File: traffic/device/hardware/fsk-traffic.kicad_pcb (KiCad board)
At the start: 2 copper layers, 83 x 45.5 mm, 49 parts, among them J1 JTAG, J2 USB_C, J3 Molex 5569-04A1, J4 Molex 5569-04A1, J5 Molex 5569-04A1, Q1 MMBT5551, Q2 AO3401A, Q3 MMBT5551, Q4 AO3401A, U1 XC6206P332MR, U2 MT3608, U3 STM32F070F6Px, U4 LTV-817S, U5 LTV-817S, Y1 12MHz

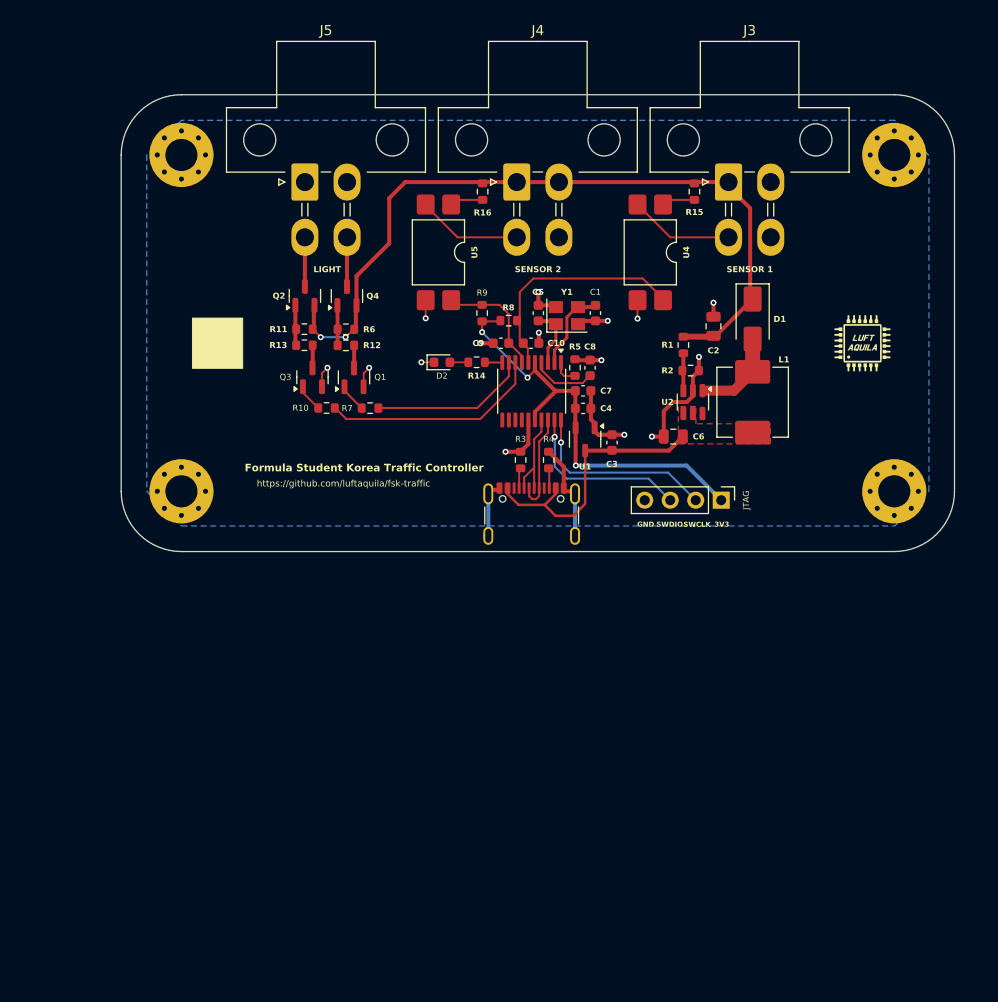
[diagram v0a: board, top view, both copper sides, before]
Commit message: impl: schematic and pcb layout
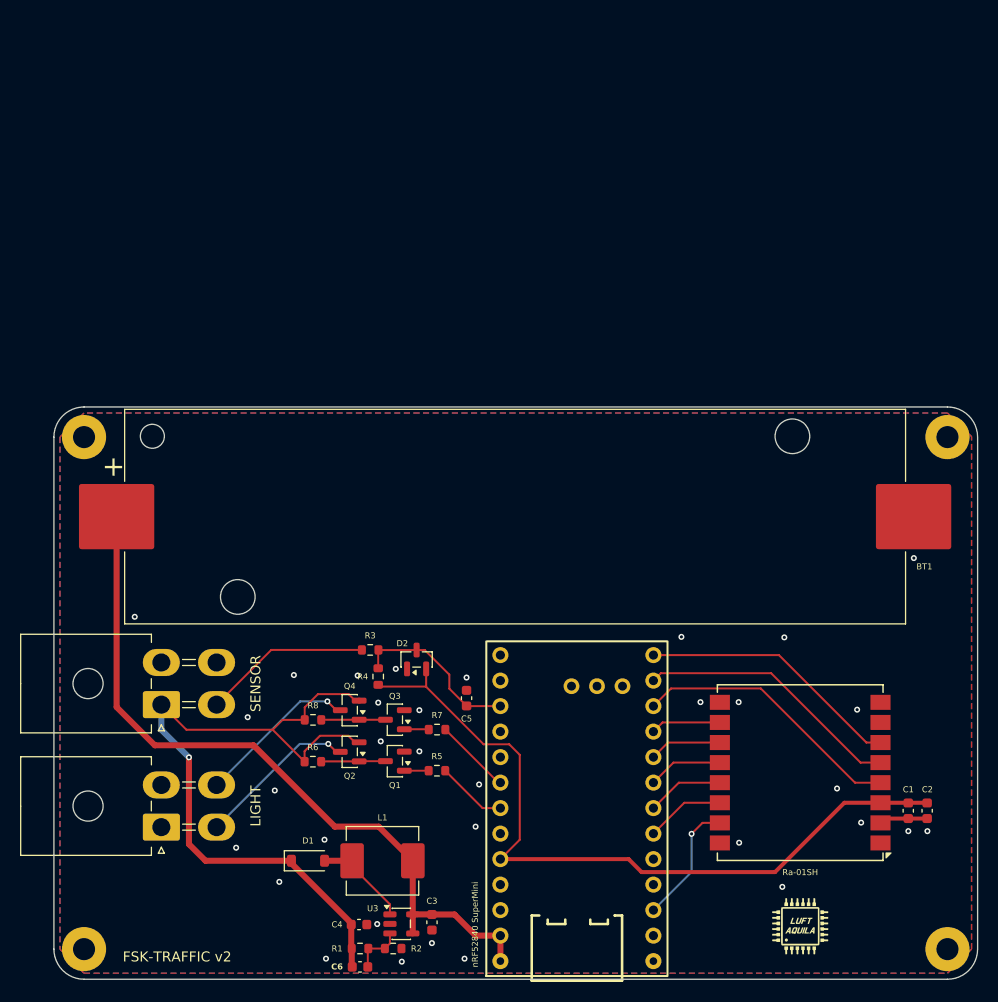
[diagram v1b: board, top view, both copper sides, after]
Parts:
- removed C10, C9: 470nF, Capacitor_SMD:C_0603_1608Metric
- removed C7, C8: 100nF, Capacitor_SMD:C_0603_1608Metric
- removed the G*** at (176.6, 104.6)
- removed J3, J4, J5: Molex 5569-04A1, Connector_Molex:Molex_Mini-Fit_Jr_5569-04A1_2x02_P4.20mm_Horizontal
- removed R10, R14: 1k, Resistor_SMD:R_0603_1608Metric
- removed R11: 10k, Resistor_SMD:R_0603_1608Metric
- removed R12, R13: 15k, Resistor_SMD:R_0603_1608Metric
- removed R15, R16: 2k, Resistor_SMD:R_0603_1608Metric
- removed R9: 3.3k, Resistor_SMD:R_0603_1608Metric
- removed the REF** at (108.7, 85.9)
- removed the REF** at (179.7, 85.9)
- removed the REF** at (108.7, 119.4)
- removed the REF** at (179.7, 119.4)
- removed U4, U5: LTV-817S, Package_DIP:SMDIP-4_W9.53mm
- removed Y1: 12MHz, Crystal:Crystal_SMD_3225-4Pin_3.2x2.5mm
- added BT1: 18650, Battery:BatteryHolder_Keystone_1042_1x18650, F.Cu at (141.9, 121.9)
- added G***: LOGO, parts:luftaquila, F.Cu at (170.3, 162.7)
- added REF**: MountingHole_2.2mm_M2_Pad, MountingHole:MountingHole_2.2mm_M2_Pad, F.Cu at (99.0, 165.0)
- added REF**: MountingHole_2.2mm_M2_Pad, MountingHole:MountingHole_2.2mm_M2_Pad, F.Cu at (185.0, 165.0)
- added REF**: MountingHole_2.2mm_M2_Pad, MountingHole:MountingHole_2.2mm_M2_Pad, F.Cu at (99.0, 114.0)
- added REF**: MountingHole_2.2mm_M2_Pad, MountingHole:MountingHole_2.2mm_M2_Pad, F.Cu at (185.0, 114.0)
- C1: value 20pF -> 100nF
- C2: value 22uF -> 10uF; footprint Capacitor_SMD:C_0805_2012Metric -> Capacitor_SMD:C_0603_1608Metric
- C3, C4: value 1uF -> 10uF
- C5: value 20pF -> 100pF
- C6: value 22uF -> 47pF; footprint Capacitor_SMD:C_0805_2012Metric -> Capacitor_SMD:C_0603_1608Metric
- D1: value SS34 -> B5819W; footprint Diode_SMD:D_SMA -> Diode_SMD:D_SOD-123
- D2: value LED -> BAT54S; footprint LED_SMD:LED_0603_1608Metric -> Package_TO_SOT_SMD:SOT-23
- J1: value JTAG -> SENSOR; footprint Connector_PinHeader_2.54mm:PinHeader_1x04_P2.54mm_Vertical -> Connector_Molex:Molex_Mini-Fit_Jr_5569-04A2_2x02_P4.20mm_Horizontal
- J2: value USB_C -> LIGHT; footprint Connector_USB:USB_C_Receptacle_GCT_USB4105-xx-A_16P_TopMnt_Horizontal -> Connector_Molex:Molex_Mini-Fit_Jr_5569-04A2_2x02_P4.20mm_Horizontal
- L1: footprint Inductor_SMD:L_Changjiang_FXL0630 -> Inductor_SMD:L_Sunlord_MWSA0603S
- Q1, Q3: value MMBT5551 -> MMBT3904
- Q2, Q4: value AO3401A -> MMBT3906
- R1: value 51k -> 1M
- R2: value 1.8k -> 110k
- R3: value 5.1k -> 330
- R4: value 5.1k -> 4.7k
- R7: value 1k -> 10k
- R8: value 3.3k -> 10k
- U1: value XC6206P332MR -> nRF52840 SuperMini; footprint Package_TO_SOT_SMD:SOT-23-3 -> lib:SuperMini_NRF52840
- U2: value MT3608 -> Ra-01SH; footprint Package_TO_SOT_SMD:SOT-23-6 -> RF_Module:Ai-Thinker-Ra-01-LoRa
- U3: value STM32F070F6Px -> TPS61040DBV; footprint Package_SO:TSSOP-20_4.4x6.5mm_P0.65mm -> Package_TO_SOT_SMD:SOT-23-5
- moved D1 69.8 mm to (121.3, 156.2), turned to 0 degrees
- moved R1 68.2 mm to (126.5, 164.9), turned to 0 degrees
- moved R2 64.7 mm to (129.8, 164.9)
- moved C6 61.3 mm to (126.5, 166.8), turned to 0 degrees
- moved J1 59.4 mm to (106.7, 140.7), turned to 90 degrees
- moved L1 58.7 mm to (128.7, 156.2), turned to 180 degrees
- moved C1 58.5 mm to (181.1, 151.2)
- moved C4 56.0 mm to (126.4, 162.6)
- moved U3 54.6 mm to (130.6, 162.5), turned to 0 degrees
- moved C2 52.7 mm to (183.0, 151.2), turned to -90 degrees
- moved U1 52.4 mm to (155.7, 166.2), turned to 180 degrees
- moved C3 51.0 mm to (133.7, 162.3), turned to -90 degrees
- moved J2 47.6 mm to (106.7, 152.8), turned to 90 degrees
- moved Q2 45.6 mm to (125.5, 145.3), turned to 180 degrees
- moved R8 44.3 mm to (121.8, 142.2), turned to 0 degrees
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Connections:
- C1 pad 1: OSC_IN -> +3.3V
- C2 pad 1: 18V -> +3.3V
- C3 pad 1: +5V -> +BATT
- C4 pad 1: +3V3 -> +12V
- C5 pad 1: OSC_OUT -> /SENSOR
- C6 pad 1: +5V -> +12V
- C6 pad 2: GND -> Net-(U3-FB)
- D1 pad 1: 18V -> +12V
- D2 pad 2: Net-(D2-A) -> +3.3V
- J1 pad 1: +3V3 -> +12V
- J1 pad 2: SWCLK -> unconnected-(J1-Pin_2-Pad2)
- J1 pad 3: SWDIO -> /SENSE
- L1 pad 1: +5V -> +BATT
- Q2 pad 1: Net-(Q2-G) -> Net-(Q1-C)
- Q2 pad 2: 18V -> +12V
- Q4 pad 1: Net-(Q4-G) -> Net-(Q3-C)
- Q4 pad 2: 18V -> +12V
- R1 pad 1: 18V -> +12V
- R1 pad 2: Net-(U2-FB) -> Net-(U3-FB)
- R2 pad 1: Net-(U2-FB) -> Net-(U3-FB)
- R3 pad 1: GND -> /SENSE
- R3 pad 2: Net-(J2-CC1) -> /SENSOR
- R4 pad 1: GND -> /SENSOR
- R4 pad 2: Net-(J2-CC2) -> +3.3V
- R5 pad 1: GND -> Net-(Q1-B)
- R5 pad 2: BOOT -> /RED
- R6 pad 1: Net-(Q4-G) -> +12V
- R6 pad 2: 18V -> Net-(Q1-C)
- R7 pad 1: Net-(Q1-B) -> Net-(Q3-B)
- R7 pad 2: GREEN -> /GREEN
- R8 pad 1: SENS1 -> +12V
- R8 pad 2: +3V3 -> Net-(Q3-C)
- U1 pad 1: GND -> unconnected-(U1-P0.06-Pad1)_1
- U1 pad 2: +3V3 -> /NSS
- U1 pad 3: +5V -> GND
- U2 pad 1: Net-(D1-A) -> unconnected-(U2-ANT-Pad1)
- U2 pad 3: Net-(U2-FB) -> +3.3V
- U2 pad 4: +5V -> /NRST
- U2 pad 5: +5V -> /TXEN
- U2 pad 6: unconnected-(U2-NC-Pad6) -> /DIO1
- U3 pad 1: BOOT -> Net-(D1-A)
- U3 pad 2: OSC_IN -> GND
- U3 pad 3: OSC_OUT -> Net-(U3-FB)
- U3 pad 4: NRST -> +BATT
- U3 pad 5: +3V3 -> +BATT
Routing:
- net 18V: track 78.2 -> 0.00 mm, vias 2 -> 0
- net +3.3V: track 0.00 -> 76.3 mm
- net +BATT: track 0.00 -> 74.2 mm
- net +12V: track 0.00 -> 74.1 mm, vias 0 -> 1
- net GND: track 60.3 -> 4.82 mm, vias 15 -> 33
- net +3V3: track 44.3 -> 0.00 mm, vias 3 -> 0
- net +5V: track 27.5 -> 0.00 mm
- net /NRST: track 0.00 -> 26.5 mm
- net /TXEN: track 0.00 -> 25.9 mm
- net /DIO1: track 0.00 -> 25.5 mm
- net SENS1: track 23.7 -> 0.00 mm
- net RED: track 22.0 -> 0.00 mm
- net SWCLK: track 19.3 -> 0.00 mm, vias 1 -> 0
- net SWDIO: track 17.5 -> 0.00 mm, vias 1 -> 0
- net /SENSOR: track 0.00 -> 17.1 mm
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- added copper zone on F.Cu, net GND
- removed copper zone on F.Cu, net +5V
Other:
- board size 83 x 45.5 mm -> 92 x 57 mm
- board text added: "FSK-TRAFFIC v2"
- board text removed: "3V3"
- board text removed: "Formula Student Korea Traffic Controller"
- board text removed: "GND"
- board text removed: "JLCPCB QR PLACEHOLDER"
- board text removed: "LIGHT"
- board text removed: "SENSOR 1"
- board text removed: "SENSOR 2"
- board text removed: "SWCLK"
- board text removed: "SWDIO"
- board text removed: "https://github.com/luftaquila/fsk-traffic"
